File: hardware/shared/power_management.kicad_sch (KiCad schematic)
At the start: 0 parts

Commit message: more kicad work
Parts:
- added C1, C11, C2: 1uF, Capacitor_SMD:C_0402_1005Metric, symbol Device:C
- added C10, C12, C13, C14, C4, C5, C7, C8, C9: 10uF, Capacitor_SMD:C_0603_1608Metric, symbol Device:C
- added C3: 4.7uF, Capacitor_SMD:C_0603_1608Metric, symbol Device:C
- added C6: 100nF, Capacitor_SMD:C_0402_1005Metric, symbol Device:C
- added D1: RED err, LED_SMD:LED_0603_1608Metric, symbol Device:LED
- added D2: GREEN chg, LED_SMD:LED_0603_1608Metric, symbol Device:LED
- added J3: USB4720-03-A, obc:GCT_USB4720-03-A_REVA, symbol obc:USB4720-03-A
- added J4: BT1 1S Li-Po, Connector_JST:JST_PH_S2B-PH-K_1x02_P2.00mm_Horizontal, symbol Connector_Generic:Conn_01x02
- added L1, L2, L3: 2.2uH, Inductor_SMD:L_Murata_DFE201610P, symbol Device:L
- added R6: 10k 1%, Resistor_SMD:R_0402_1005Metric, symbol Device:R
- added R7: 300k 1%, Resistor_SMD:R_0402_1005Metric, symbol Device:R
- added SW5: PWR, Button_Switch_SMD:SW_SPST_EVQP7C, symbol Switch:SW_Push
- added U2: NPM1300-CAAA-R, obc:BGA35N44X41P5X7_237X307X51, symbol obc:NPM1300-CAAA-R
- added U7: TPS610997, symbol obc:TPS610997
- added U8: USBLC6-2SC6, Package_TO_SOT_SMD:SOT-23-6, symbol Power_Protection:USBLC6-2SC6
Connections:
- new net: SW5.2, U2.D4 (SHPHLD)
- new net: L3.2, U7.5 (SW)
- new net: L1.1, U2.B7 (SW1)
- new net: D1.1 (K), U2.A1 (LED0)
- new net: D2.1 (K), U2.A2 (LED1)
- new net: R6.1, U2.D3 (NTC)
- new net: L2.1, U2.D7 (SW2)
- new net: R7.1, U2.E1 (VSET2)
- new net +1V8_MAG: C10.1, C9.1, U2.A4 (LSOUT1/VOUTLDO1)
- new net +3V3: C6.1, C8.1, L2.2, U2.B4 (LSIN1/VINLDO1), U2.B5 (LSIN2/VINLDO2), U2.C6 (VOUT2), U2.E4 (VDDIO)
- new net +3V3_GPS: C11.1, U2.A5 (LSOUT2/VOUTLDO2)
- new net +3V3_SD: C7.1, L1.2, U2.B6 (VOUT1)
- new net +5V_DISP: C13.1, C14.1, U7.2 (VOUT)
- new net DISP_5V_EN: U7.4 (EN)
- new net GND: C1.2, C10.2, C11.2, C12.2, C13.2, C14.2, C2.2, C3.2, C4.2, C5.2, C6.2, C7.2, C8.2, C9.2, J3.A1_B12 (GND_A), J3.B1_A12 (GND_B), J3.SH1 (SHIELD), J3.SH2 (SHIELD), J3.SH3 (SHIELD), J3.SH4 (SHIELD), J3.SH5 (SHIELD), J3.SH6 (SHIELD), J4.2 (Pin_2), R6.2, R7.2, SW5.1, U2.A6 (AVSS), U2.A7 (PVSS1), U2.E2 (VSET1), U2.E7 (PVSS2), U7.1 (GND), U7.3 (FB), U7.7 (PAD), U8.2 (GND)
- new net PMIC_INT: U2.C4 (GPIO3)
- new net SCL: U2.E3 (SCL)
- new net SDA: U2.E5 (SDA)
- new net USB_CC1: J3.A5 (CC1), U2.D5 (CC1)
- new net USB_CC2: J3.B5 (CC2), U2.B3 (CC2)
- new net USB_DM: J3.A7 (DN1), J3.B7 (DN2), U8.1 (I/O1), U8.6 (I/O1)
- new net USB_DP: J3.A6 (DP1), J3.B6 (DP2), U8.3 (I/O2), U8.4 (I/O2)
- new net VBAT: C3.1, J4.1 (Pin_1), U2.D1 (VBAT), U2.D2 (VBAT)
- new net VBUS: C1.1, J3.A4_B9 (VBUS_A), J3.B4_A9 (VBUS_B), U2.B1 (VBUS), U2.B2 (VBUS), U8.5 (VBUS)
- new net VBUS_MCU: C2.1, U2.C3 (VBUSOUT)
- new net VSYS: C12.1, C4.1, C5.1, D1.2 (A), D2.2 (A), L3.1, U2.C1 (VSYS), U2.C2 (VSYS), U2.C7 (PVDD), U7.6 (VIN)
- no-connect marks 0 -> 6
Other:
- note added: "5V DISPLAY BOOST — TPS610997"
- note added: "BATTERY"
- note added: "ERC FLAGS"
- note added: "PVDD"
- note added: "USB-C"
- note added: "VBUSOUT"
- note added: "VSET2=300k -> BUCK2 3.3V at startup (main rail). VSET1=GND -> BUCK1 OFF at startup; fw sets 3.3V, enables only to mount SD (power gate). LDSW1 = LDO 1.8V from +3V3 -> BMM350 VDD. LDSW2 = load switch +3V3 -> +3V3_GPS. Both OFF at boot - fw enables via I2C (0x6B). Charge current set in fw; NTC fixed 10k (no pack thermistor) -> disable NTC monitor or treat 25C. LED0 = charger error, LED1 = charging 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"
- note added: "nPM1300 — CHARGER + BUCKS + LDSW"
- note added: "pack NTC: n/a (R6 fixed)"
- company: (none) -> OpenBikeComputer
- title: (none) -> Power Management

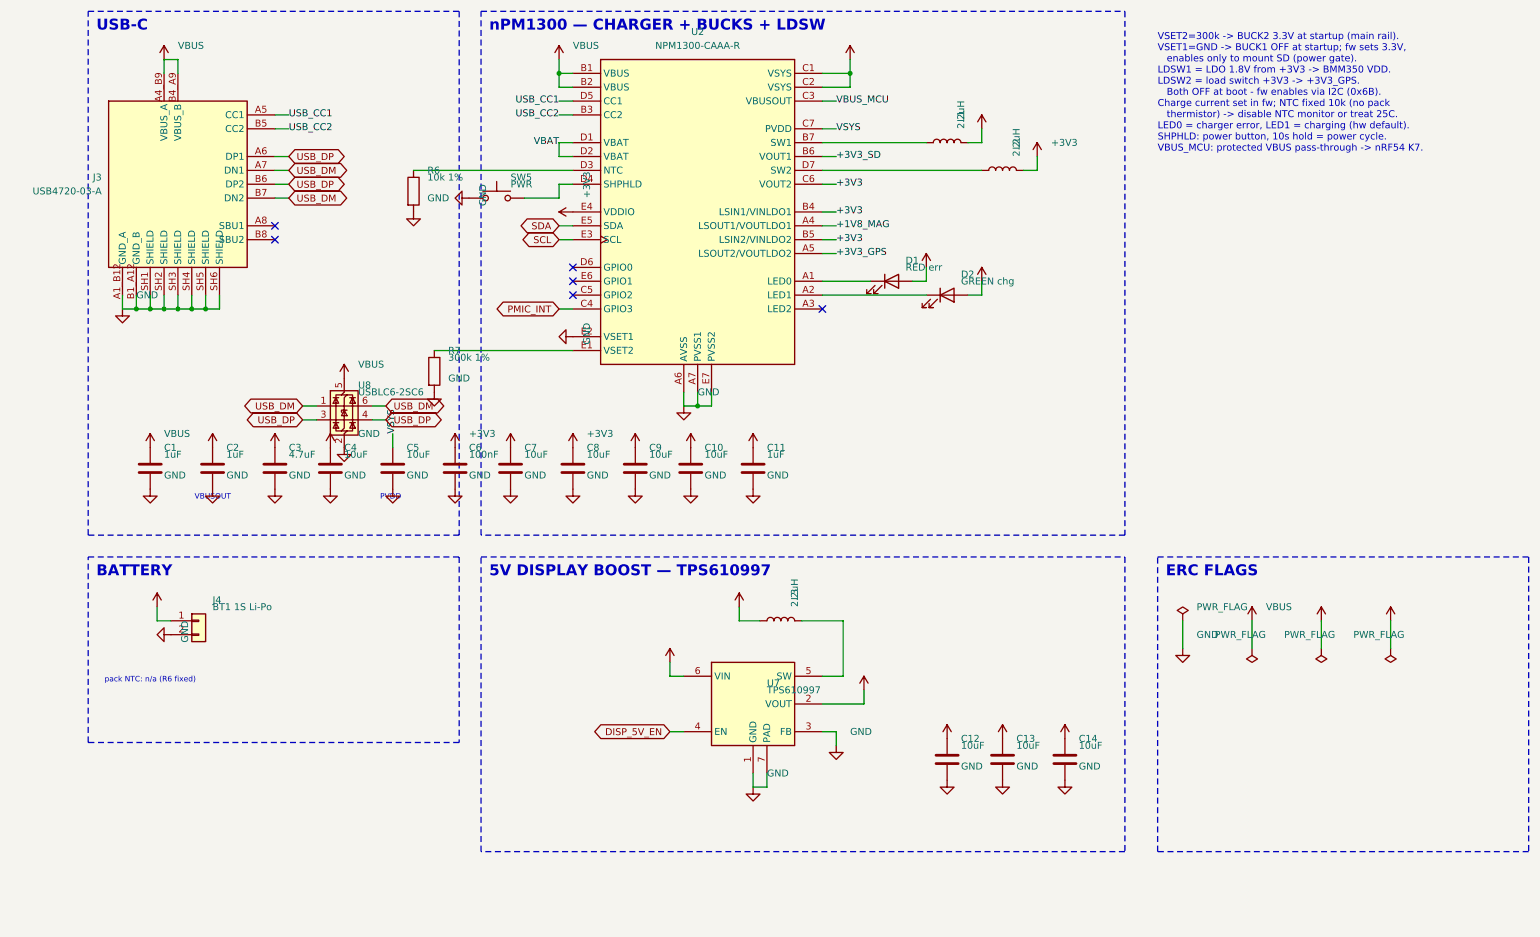
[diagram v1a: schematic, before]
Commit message: more pcb work - add baseboard remove Proto
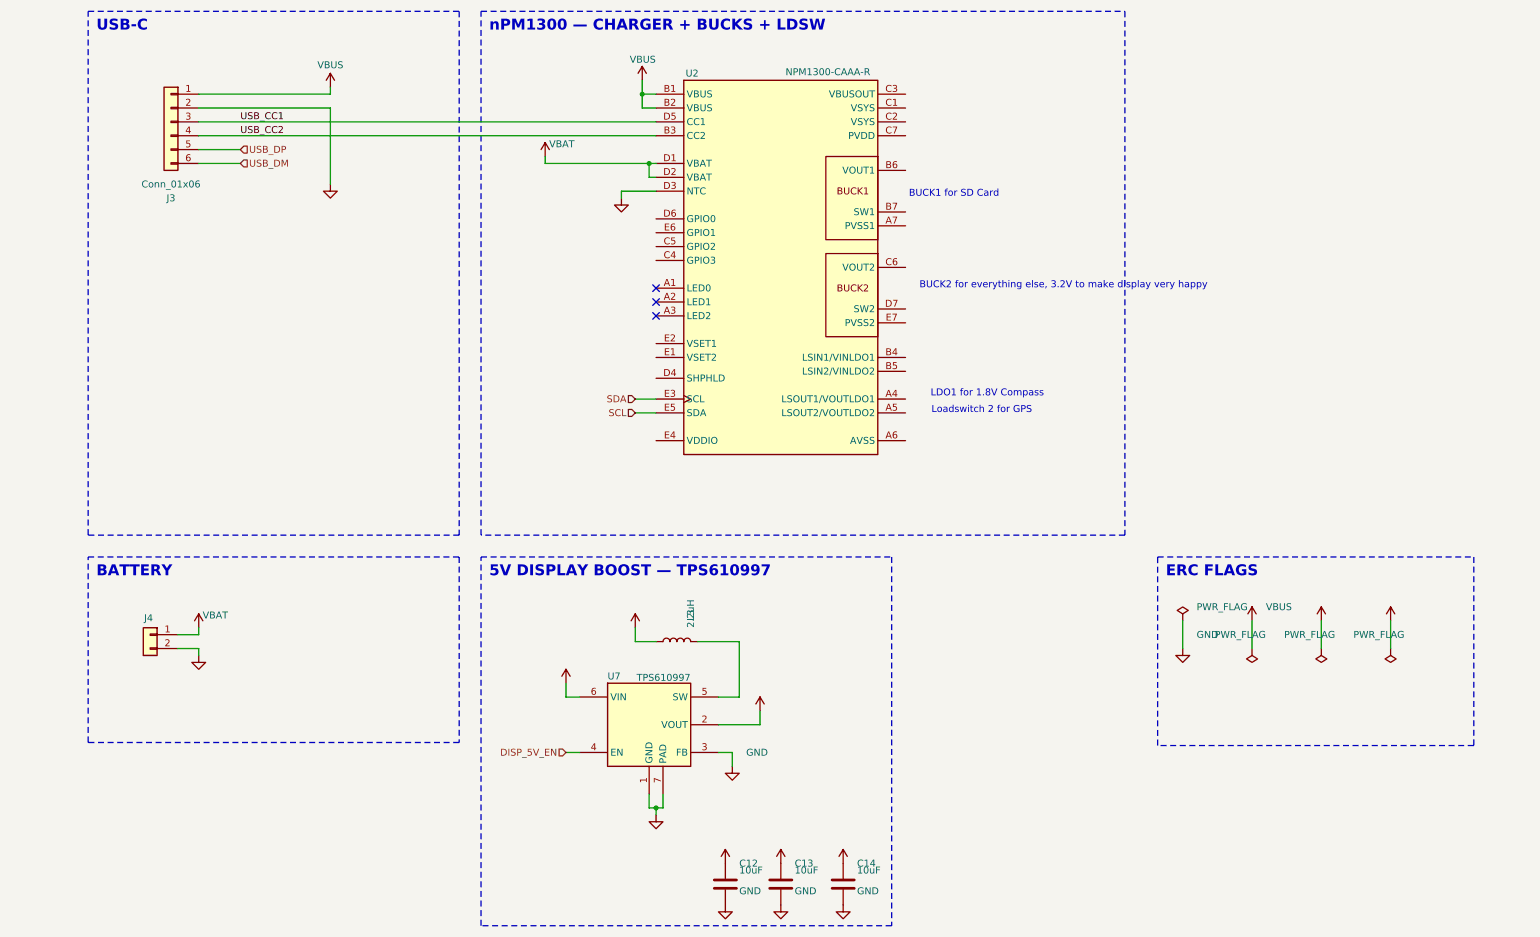
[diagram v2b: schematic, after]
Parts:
- removed C1, C11, C2: 1uF, Capacitor_SMD:C_0402_1005Metric, symbol Device:C
- removed C10, C4, C5, C7, C8, C9: 10uF, Capacitor_SMD:C_0603_1608Metric, symbol Device:C
- removed C3: 4.7uF, Capacitor_SMD:C_0603_1608Metric, symbol Device:C
- removed C6: 100nF, Capacitor_SMD:C_0402_1005Metric, symbol Device:C
- removed D1: RED err, LED_SMD:LED_0603_1608Metric, symbol Device:LED
- removed D2: GREEN chg, LED_SMD:LED_0603_1608Metric, symbol Device:LED
- removed J3: USB4720-03-A, obc:GCT_USB4720-03-A_REVA, symbol obc:USB4720-03-A
- removed L1, L2: 2.2uH, Inductor_SMD:L_Murata_DFE201610P, symbol Device:L
- removed R6: 10k 1%, Resistor_SMD:R_0402_1005Metric, symbol Device:R
- removed R7: 300k 1%, Resistor_SMD:R_0402_1005Metric, symbol Device:R
- removed SW5: PWR, Button_Switch_SMD:SW_SPST_EVQP7C, symbol Switch:SW_Push
- removed U8: USBLC6-2SC6, Package_TO_SOT_SMD:SOT-23-6, symbol Power_Protection:USBLC6-2SC6
- added J3: Conn_01x06, symbol Connector_Generic:Conn_01x06
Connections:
- net GND: now also U2.D3 (NTC), J3.2 (Pin_2); no longer U2.A6 (AVSS), U2.A7 (PVSS1), U2.E2 (VSET1), U2.E7 (PVSS2)
- net SCL: now also U2.E5 (SDA); no longer U2.E3 (SCL)
- net SDA: now also U2.E3 (SCL); no longer U2.E5 (SDA)
- net USB_CC1: now also J3.3 (Pin_3)
- net USB_CC2: now also J3.4 (Pin_4)
- net USB_DM: now also J3.6 (Pin_6)
- net USB_DP: now also J3.5 (Pin_5)
- net VBUS: now also J3.1 (Pin_1)
- net VSYS: no longer U2.C1 (VSYS), U2.C2 (VSYS), U2.C7 (PVDD)
- net +1V8_MAG: no longer names the net of U2.A4 (LSOUT1/VOUTLDO1)
- removed net +3V3: U2.B4 (LSIN1/VINLDO1), U2.B5 (LSIN2/VINLDO2), U2.C6 (VOUT2), U2.E4 (VDDIO)
- net +3V3_GPS: no longer names the net of U2.A5 (LSOUT2/VOUTLDO2)
- net +3V3_SD: no longer names the net of U2.B6 (VOUT1)
- net PMIC_INT: no longer names the net of U2.C4 (GPIO3)
- net VBUS_MCU: no longer names the net of U2.C3 (VBUSOUT)
- no-connect marks 6 -> 3
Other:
- note added: "BUCK1 for SD Card"
- note added: "BUCK2 for everything else, 3.2V to make display very happy"
- note added: "LDO1 for 1.8V Compass"
- note added: "Loadswitch 2 for GPS"
- note removed: "PVDD"
- note removed: "VBUSOUT"
- note removed: "VSET2=300k -> BUCK2 3.3V at startup (main rail). VSET1=GND -> BUCK1 OFF at startup; fw sets 3.3V, enables only to mount SD (power gate). LDSW1 = LDO 1.8V from +3V3 -> BMM350 VDD. LDSW2 = load switch +3V3 -> +3V3_GPS. Both OFF at boot - fw enables via I2C (0x6B). Charge current set in fw; NTC fixed 10k (no pack thermistor) -> disable NTC monitor or treat 25C. LED0 = charger error, LED1 = charging 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"
- note removed: "pack NTC: n/a (R6 fixed)"
- moved on the sheet: C12, C13, C14, J4, L3, U7
